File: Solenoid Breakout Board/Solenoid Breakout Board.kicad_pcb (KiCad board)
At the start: 2 copper layers, 144.1 x 102.2 mm, 155 parts, among them J1 Solenoid In, J2 Pwr IN, J3 Pwr OUT, Q1 IRF540N, Q10 IRF540N, Q11 IRF540N, Q12 IRF540N, Q13 IRF540N, Q14 IRF540N, Q15 IRF540N, Q16 IRF540N, Q17 IRF540N, Q18 IRF540N, Q19 IRF540N, Q2 IRF540N, Q20 IRF540N, Q3 IRF540N, Q4 IRF540N, Q5 IRF540N, Q6 IRF540N, Q7 IRF540N, Q8 IRF540N, Q9 IRF540N, U1 LTV-247, U2 LTV-247, U3 LTV-247, U4 LTV-247, U5 LTV-247

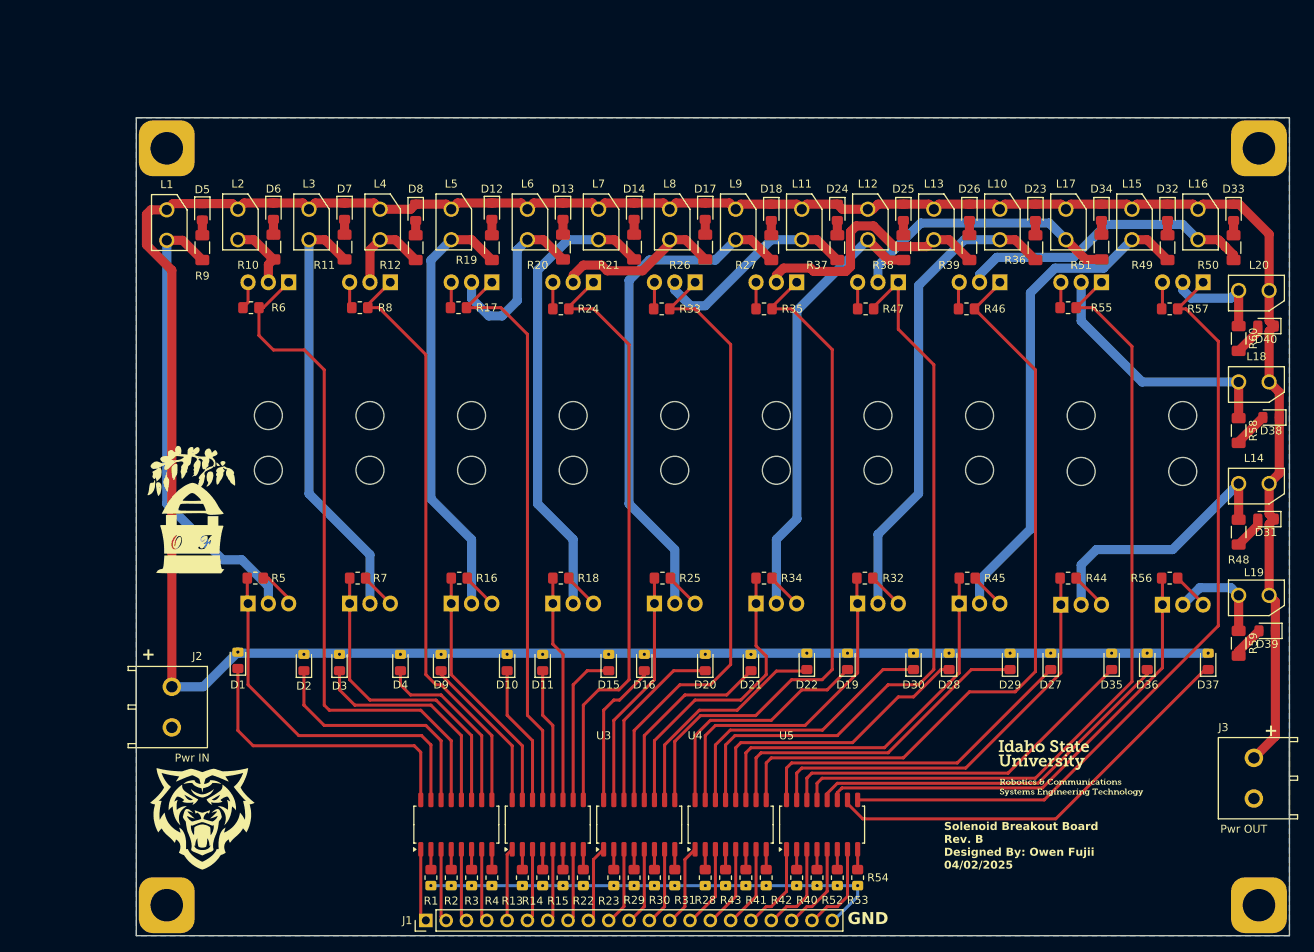
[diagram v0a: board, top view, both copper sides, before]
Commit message: added pcb sheets
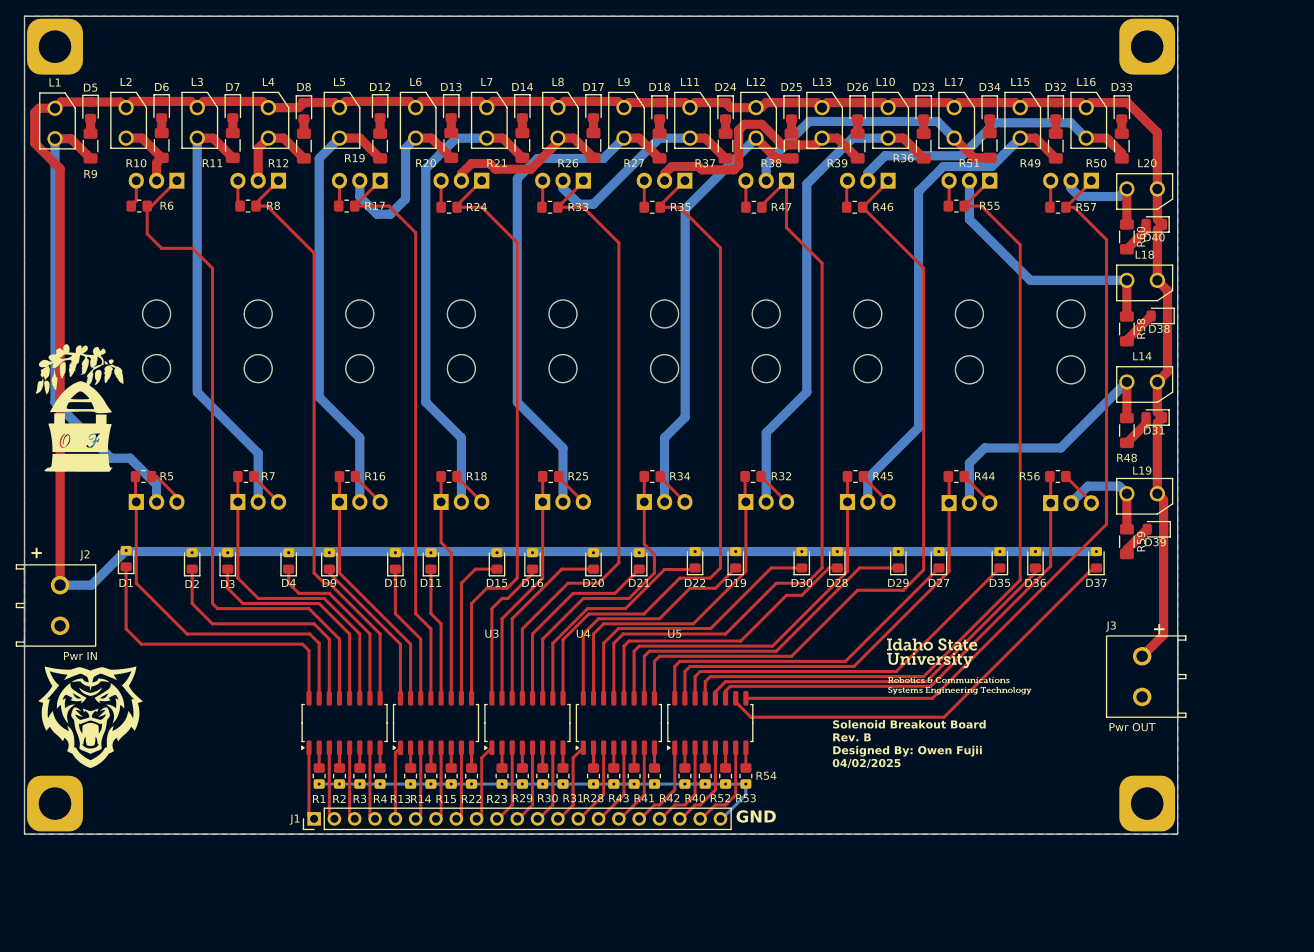
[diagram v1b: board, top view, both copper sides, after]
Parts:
- moved D33 18.9 mm to (167.6, 52.5)
- moved R50 18.9 mm to (167.6, 56.9)
- moved D10 18.9 mm to (76.8, 108.7)
- moved D13 18.9 mm to (83.8, 52.3)
- moved D14 18.9 mm to (92.7, 52.3)
- moved D22 18.9 mm to (114.3, 108.6)
- moved R20 18.9 mm to (83.8, 56.8)
- moved R21 18.9 mm to (92.7, 56.8)
- moved D24 18.9 mm to (118.1, 52.5)
- moved D25 18.9 mm to (126.4, 52.5)
- moved J2 18.9 mm to (34.9, 114.3)
- moved L20 18.9 mm to (172.1, 62.2)
- moved Q3 18.9 mm to (57.1, 101.4)
- moved Q4 18.9 mm to (62.2, 61.2)
- moved R37 18.9 mm to (118.1, 56.9)
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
